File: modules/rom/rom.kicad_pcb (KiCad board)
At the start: 2 copper layers, 126.8 x 77 mm, 65 parts, among them J14 Conn_02x05_Odd_Even, K1 4PDT, K2 4PDT, SW1 SW_DIP_x04, SW2 SW_DIP_x04, SW3 SW_DIP_x04, SW4 SW_DIP_x04, SW5 SW_DIP_x04, SW6 SW_DIP_x04, SW7 SW_DIP_x04, SW8 SW_DIP_x04

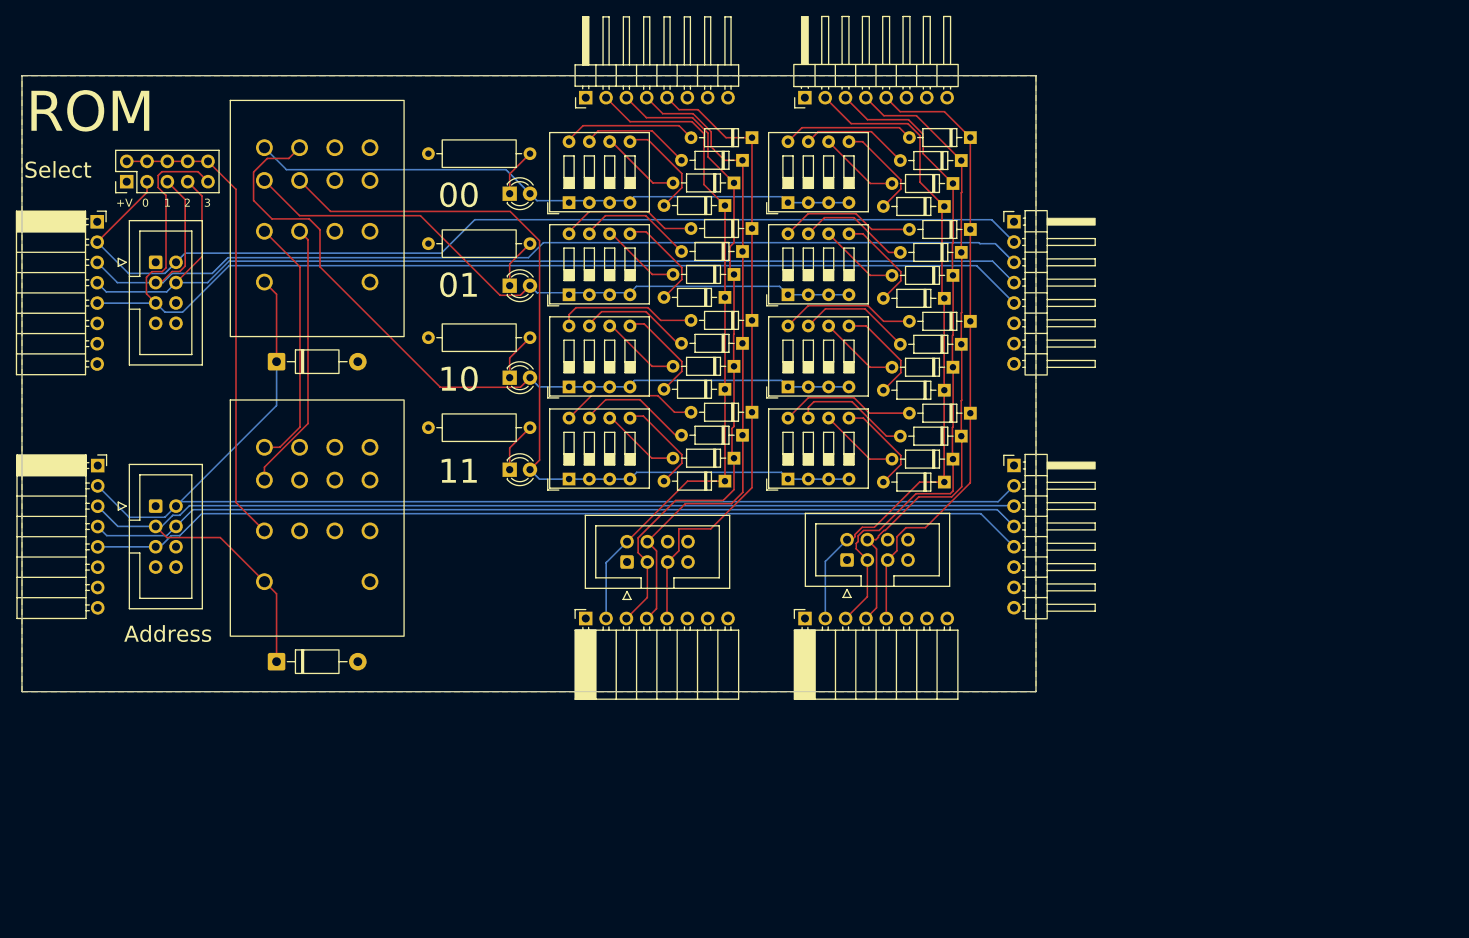
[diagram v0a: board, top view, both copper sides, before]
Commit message: Updated actions
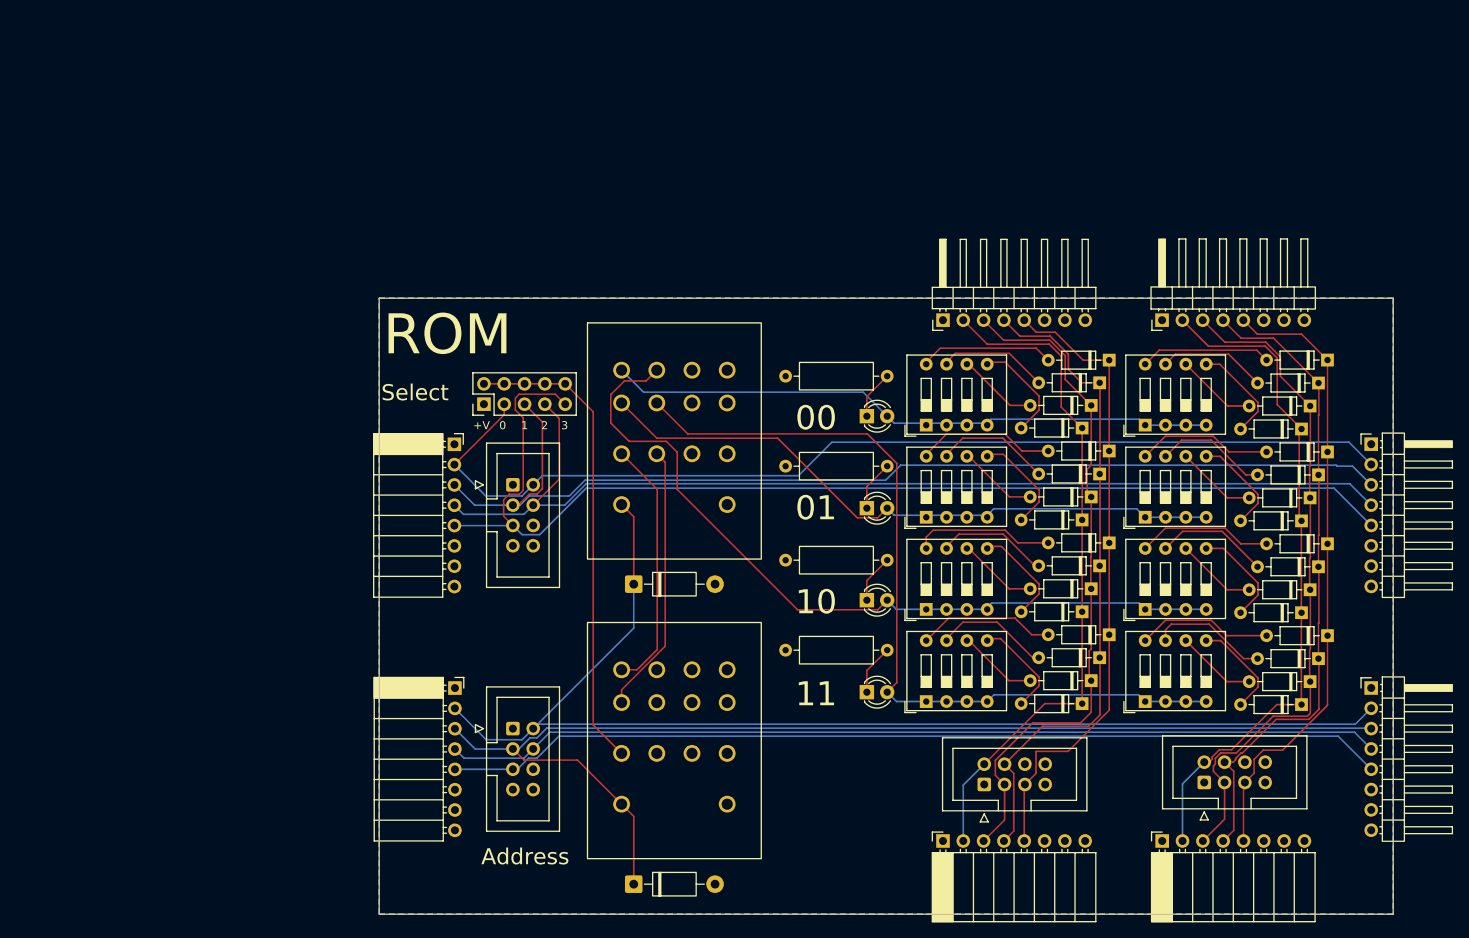
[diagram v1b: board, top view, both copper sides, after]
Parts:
- moved D1 52.6 mm to (137.1, 66.8)
- moved D2 52.6 mm to (137.1, 78.3)
- moved D3 52.6 mm to (137.1, 89.8)
- moved D4 52.6 mm to (137.1, 101.3)
- moved D12 52.6 mm to (164.0, 68.3)
- moved D13 52.6 mm to (167.4, 71.2)
- moved D14 52.6 mm to (166.2, 74.0)
- moved D16 52.6 mm to (164.0, 79.8)
- moved D18 52.6 mm to (166.2, 85.5)
- moved D20 52.6 mm to (164.0, 91.3)
- moved D21 52.6 mm to (167.4, 94.1)
- moved D22 52.6 mm to (166.2, 97.0)
- moved D23 52.6 mm to (165.2, 99.9)
- moved D24 52.6 mm to (164.0, 102.7)
- moved D28 52.6 mm to (191.4, 68.4)
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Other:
- board text added: "Сигнал выборки"
- board text added: "Шина адреса"
- board text added: "Шина данных"
